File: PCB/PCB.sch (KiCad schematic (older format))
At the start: 20 parts, among them J1 AVR-ISP-6, SW1 SW_Push

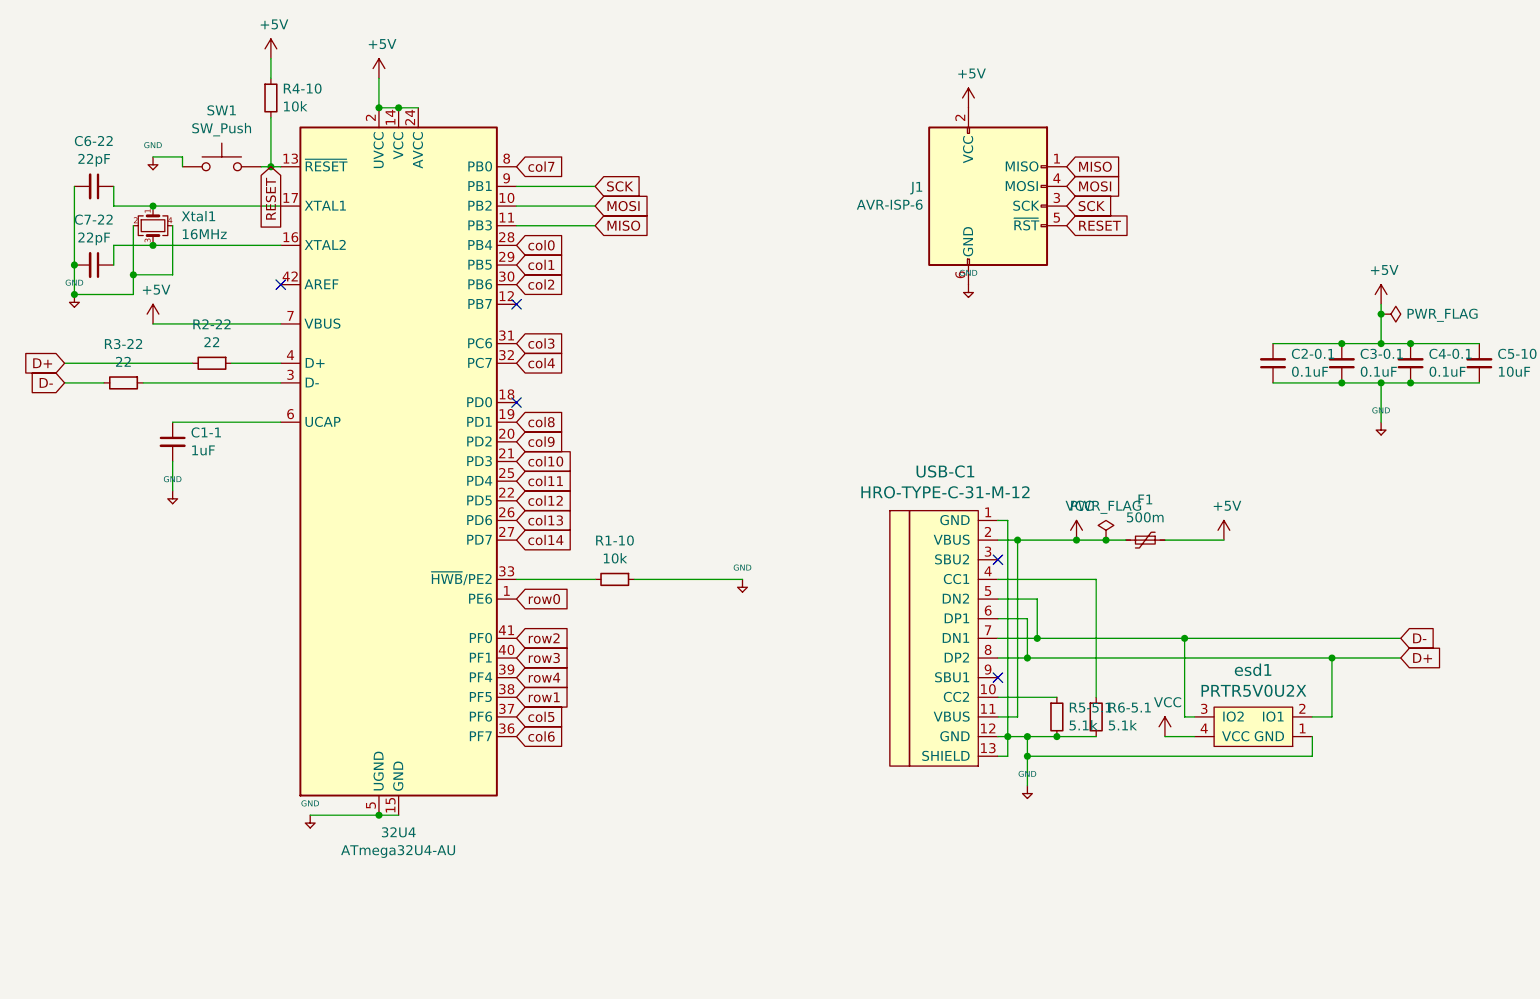
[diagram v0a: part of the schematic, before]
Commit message: pcb alignment
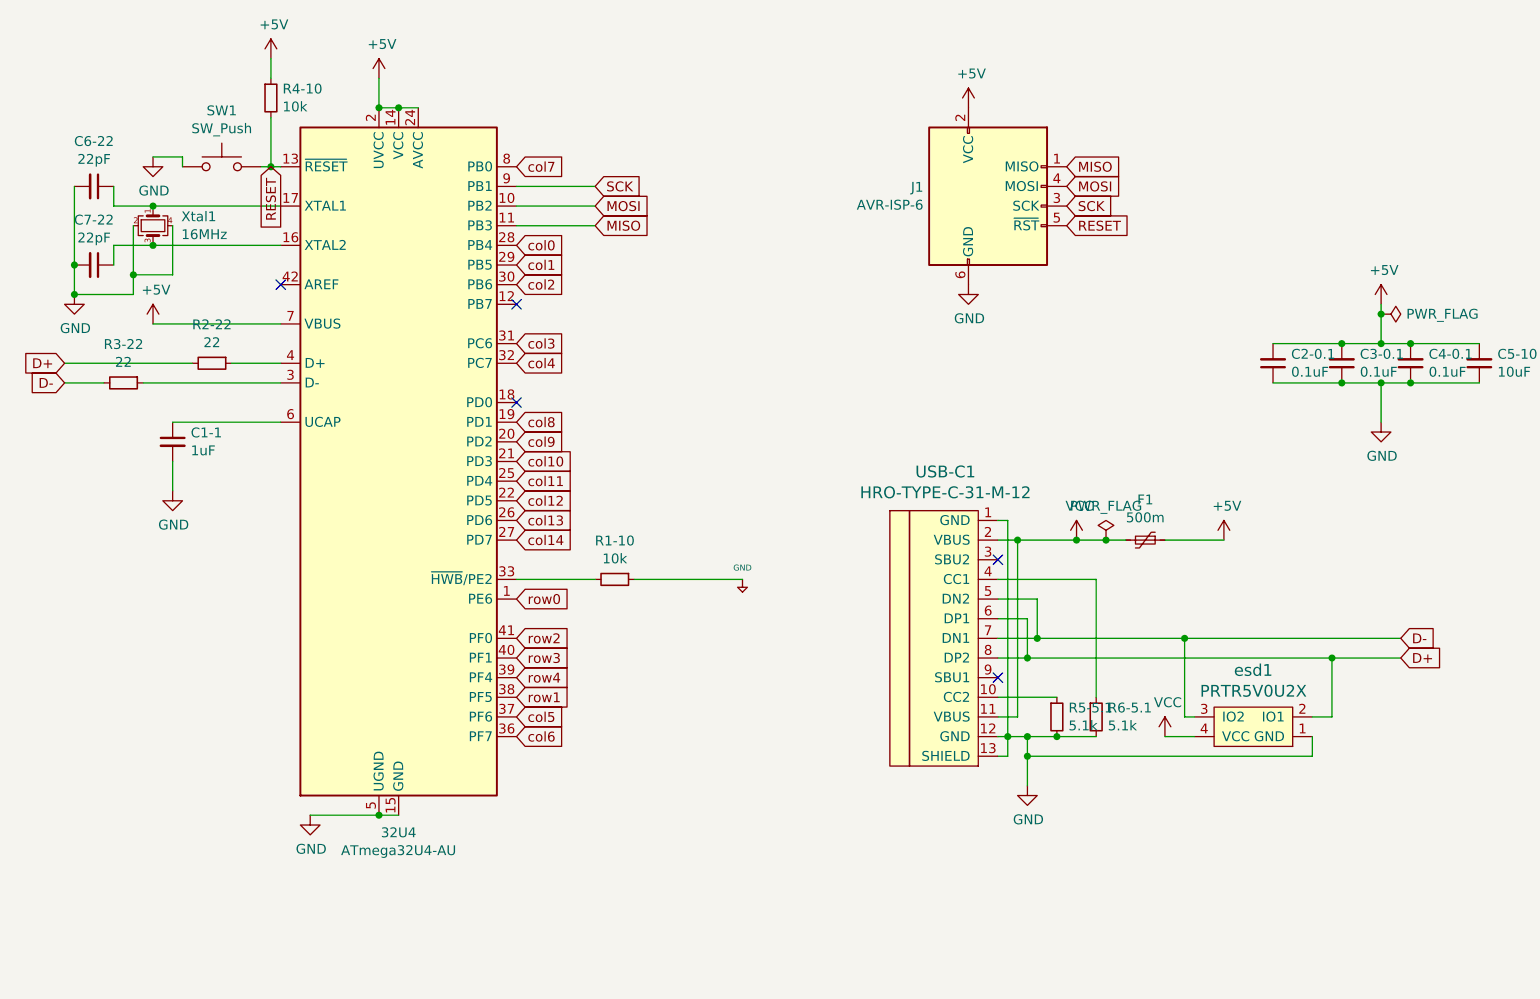
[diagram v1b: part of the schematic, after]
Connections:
- net +5V: no longer 32U4.15 (GND), 32U4.23 (GND), 32U4.35 (GND), 32U4.43 (GND), 32U4.5 (UGND), C1-1.2, C2-0.1.1, C3-0.1.1, C4-0.1.1, C5-10.1, C6-22.2, C7-22.2, J1.6 (GND), R5-5.1.2, R6-5.1.2, SW1.1, USB-C1.1 (GND), USB-C1.12 (GND), USB-C1.13 (SHIELD), Xtal1.2, Xtal1.4, esd1.1 (GND)
- new net GND: 32U4.15 (GND), 32U4.23 (GND), 32U4.35 (GND), 32U4.43 (GND), 32U4.5 (UGND), C1-1.2, C2-0.1.1, C3-0.1.1, C4-0.1.1, C5-10.1, C6-22.2, C7-22.2, J1.6 (GND), R5-5.1.2, R6-5.1.2, SW1.1, USB-C1.1 (GND), USB-C1.12 (GND), USB-C1.13 (SHIELD), Xtal1.2, Xtal1.4, esd1.1 (GND)
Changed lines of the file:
@@
 	3400 1850 3400 1700
 Connection ~ 3400 1850
-$Comp
-L keyboard_parts:GND #PWR0102
-U 1 1 61E99B0D
-P 3050 5450
-F 0 "#PWR0102" H 3050 5500 20  0001 C CNN
-F 1 "GND" H 3050 5509 30  0000 C CNN
-F 2 "" H 3050 5450 60  0000 C CNN
-F 3 "" H 3050 5450 60  0000 C CNN
-	1    3050 5450
-	1    0    0    -1
-$EndComp
 Wire Wire Line
 	3500 5450 3400 5450
@@
 F 3 "~" H 2350 3550 50  0001 C CNN
 	1    2350 3550
-	1    0    0    -1
-$EndComp
-$Comp
-L keyboard_parts:GND #PWR0104
-U 1 1 61EA46C1
-P 2350 3800
-F 0 "#PWR0104" H 2350 3850 20  0001 C CNN
-F 1 "GND" H 2350 3859 30  0000 C CNN
-F 2 "" H 2350 3800 60  0000 C CNN
-F 3 "" H 2350 3800 60  0000 C CNN
-	1    2350 3800
 	1    0    0    -1
 $EndComp
@@
 	1    0    0    -1
 $EndComp
-$Comp
-L keyboard_parts:GND #PWR0106
-U 1 1 61EAE9F7
-P 8500 3450
-F 0 "#PWR0106" H 8500 3500 20  0001 C CNN
-F 1 "GND" H 8500 3509 30  0000 C CNN
-F 2 "" H 8500 3450 60  0000 C CNN
-F 3 "" H 8500 3450 60  0000 C CNN
-	1    8500 3450
-	1    0    0    -1
-$EndComp
 Wire Wire Line
 	7950 3050 8300 3050
@@
 Wire Wire Line
 	8500 3050 8650 3050
-Wire Wire Line
-	8500 3250 8500 3450
 Connection ~ 8500 3250
 Wire Wire Line
@@
 	0    1    1    0
 $EndComp
-$Comp
-L keyboard_parts:GND #PWR0108
-U 1 1 61EBA72E
-P 1850 2800
-F 0 "#PWR0108" H 1850 2850 20  0001 C CNN
-F 1 "GND" H 1850 2859 30  0000 C CNN
-F 2 "" H 1850 2800 60  0000 C CNN
-F 3 "" H 1850 2800 60  0000 C CNN
-	1    1850 2800
-	1    0    0    -1
-$EndComp
 Wire Wire Line
 	2250 2350 2050 2350
@@
 Wire Wire Line
 	2150 2800 1850 2800
-Connection ~ 1850 2800
 Wire Wire Line
 	2350 2450 2350 2700
@@
 	1    0    0    -1
 $EndComp
-$Comp
-L keyboard_parts:GND #PWR0109
-U 1 1 61EC0936
-P 2250 2100
-F 0 "#PWR0109" H 2250 2150 20  0001 C CNN
-F 1 "GND" H 2250 2159 30  0000 C CNN
-F 2 "" H 2250 2100 60  0000 C CNN
-F 3 "" H 2250 2100 60  0000 C CNN
-	1    2250 2100
-	1    0    0    -1
-$EndComp
 Wire Wire Line
 	2900 2150 2850 2150
 Wire Wire Line
 	2400 2150 2400 2100
-Wire Wire Line
-	2400 2100 2250 2100
 $Comp
 L Device:R_Small R4-10
@@
 F 3 " ~" H 5225 1800 50  0001 C CNN
 	1    6500 2350
-	1    0    0    -1
-$EndComp
-$Comp
-L keyboard_parts:GND #PWR0111
-U 1 1 61ECC37C
-P 6400 2750
-F 0 "#PWR0111" H 6400 2800 20  0001 C CNN
-F 1 "GND" H 6400 2809 30  0000 C CNN
-F 2 "" H 6400 2750 60  0000 C CNN
-F 3 "" H 6400 2750 60  0000 C CNN
-	1    6400 2750
 	1    0    0    -1
 $EndComp
@@
 Wire Wire Line
 	6700 5050 6850 5050
-$Comp
-L keyboard_parts:GND #PWR0115
-U 1 1 61EFFBF0
-P 6700 5300
-F 0 "#PWR0115" H 6700 5350 20  0001 C CNN
-F 1 "GND" H 6700 5359 30  0000 C CNN
-F 2 "" H 6700 5300 60  0000 C CNN
-F 3 "" H 6700 5300 60  0000 C CNN
-	1    6700 5300
-	1    0    0    -1
-$EndComp
-Wire Wire Line
-	6700 5150 6700 5300
 Connection ~ 6700 5150
 $Comp
@@
 Wire Wire Line
 	7400 4050 7700 4050
+Wire Wire Line
+	6700 5150 6700 5300
+Wire Wire Line
+	2250 2100 2400 2100
+Wire Wire Line
+	8500 3250 8500 3450
+$Comp
+L power:GND #PWR?
+U 1 1 62479121
+P 8500 3450
+F 0 "#PWR?" H 8500 3200 50  0001 C CNN
+F 1 "GND" H 8505 3277 50  0000 C CNN
+F 2 "" H 8500 3450 50  0001 C CNN
+F 3 "" H 8500 3450 50  0001 C CNN
+	1    8500 3450
+	1    0    0    -1
+$EndComp
+$Comp
+L power:GND #PWR?
+U 1 1 6247C0CA
+P 2250 2100
+F 0 "#PWR?" H 2250 1850 50  0001 C CNN
+F 1 "GND" H 2255 1927 50  0000 C CNN
+F 2 "" H 2250 2100 50  0001 C CNN
+F 3 "" H 2250 2100 50  0001 C CNN
+	1    2250 2100
+	1    0    0    -1
+$EndComp
+$Comp
+L power:GND #PWR?
+U 1 1 6247D056
+P 1850 2800
+F 0 "#PWR?" H 1850 2550 50  0001 C CNN
+F 1 "GND" H 1855 2627 50  0000 C CNN
+F 2 "" H 1850 2800 50  0001 C CNN
+F 3 "" H 1850 2800 50  0001 C CNN
+	1    1850 2800
+	1    0    0    -1
+$EndComp
+Connection ~ 1850 2800
+$Comp
+L power:GND #PWR?
+U 1 1 6247E214
+P 2350 3800
+F 0 "#PWR?" H 2350 3550 50  0001 C CNN
+F 1 "GND" H 2355 3627 50  0000 C CNN
+F 2 "" H 2350 3800 50  0001 C CNN
+F 3 "" H 2350 3800 50  0001 C CNN
+	1    2350 3800
+	1    0    0    -1
+$EndComp
+$Comp
+L power:GND #PWR?
+U 1 1 6247EC26
+P 3050 5450
+F 0 "#PWR?" H 3050 5200 50  0001 C CNN
+F 1 "GND" H 3055 5277 50  0000 C CNN
+F 2 "" H 3050 5450 50  0001 C CNN
+F 3 "" H 3050 5450 50  0001 C CNN
+	1    3050 5450
+	1    0    0    -1
+$EndComp
+$Comp
+L power:GND #PWR?
+U 1 1 6247EF75
+P 6700 5300
+F 0 "#PWR?" H 6700 5050 50  0001 C CNN
+F 1 "GND" H 6705 5127 50  0000 C CNN
+F 2 "" H 6700 5300 50  0001 C CNN
+F 3 "" H 6700 5300 50  0001 C CNN
+	1    6700 5300
+	1    0    0    -1
+$EndComp
+$Comp
+L power:GND #PWR?
+U 1 1 6247FB74
+P 6400 2750
+F 0 "#PWR?" H 6400 2500 50  0001 C CNN
+F 1 "GND" H 6405 2577 50  0000 C CNN
+F 2 "" H 6400 2750 50  0001 C CNN
+F 3 "" H 6400 2750 50  0001 C CNN
+	1    6400 2750
+	1    0    0    -1
+$EndComp
 $EndSCHEMATC
